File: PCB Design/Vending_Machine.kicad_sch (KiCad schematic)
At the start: 1 part, among them P01 Main Supply

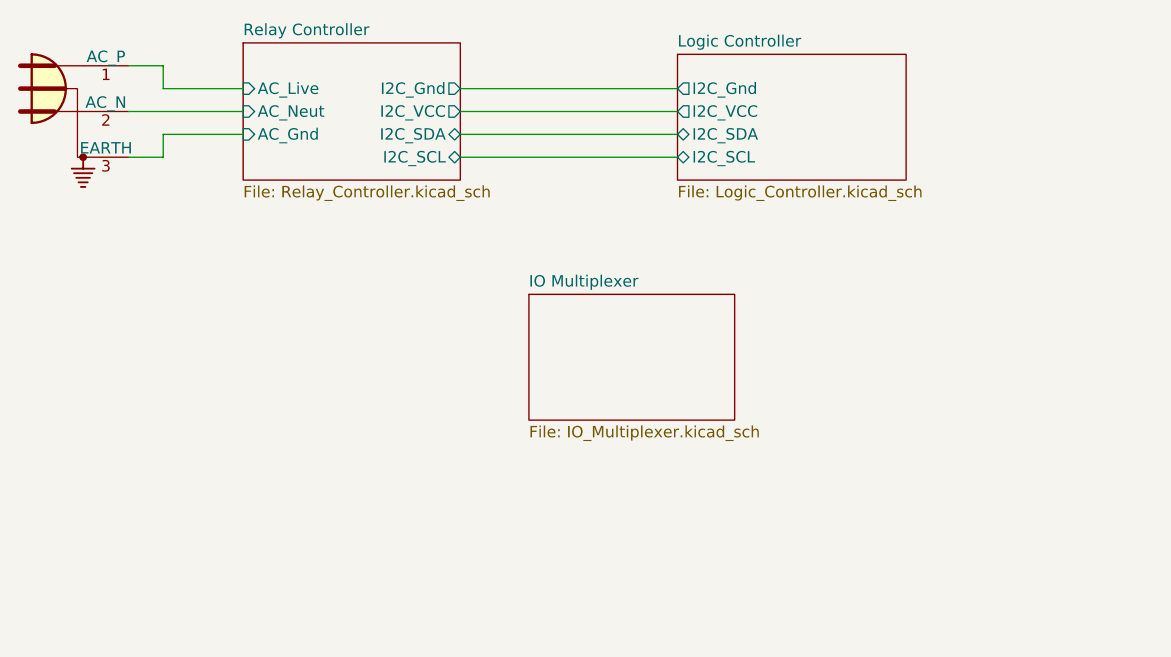
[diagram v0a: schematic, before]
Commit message: Minor Improvements
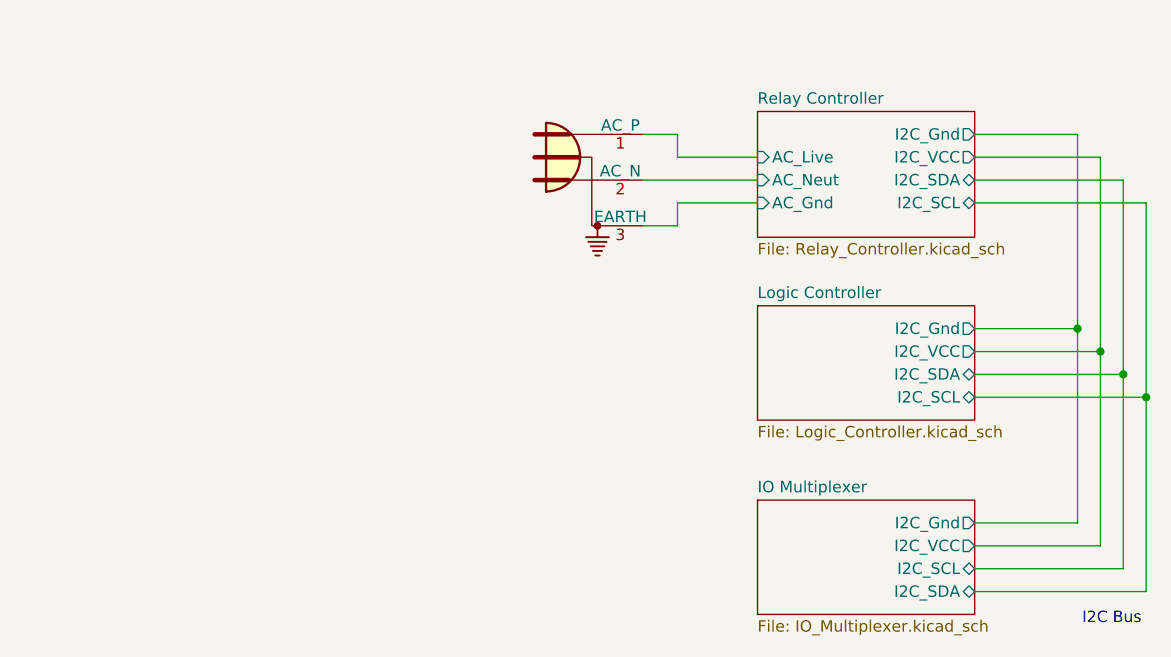
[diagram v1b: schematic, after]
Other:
- sheet IO Multiplexer ports: added I2C_Gnd, I2C_SCL, I2C_SDA, I2C_VCC; removed none
- note added: "I2C Bus"
